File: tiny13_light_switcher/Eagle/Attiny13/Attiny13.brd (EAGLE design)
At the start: 80 x 85 mm, 39 parts, among them Q4 2N7000, Q5 2N7000, Q6 2N7000, U1 ATTiny13, U2 ATTiny85

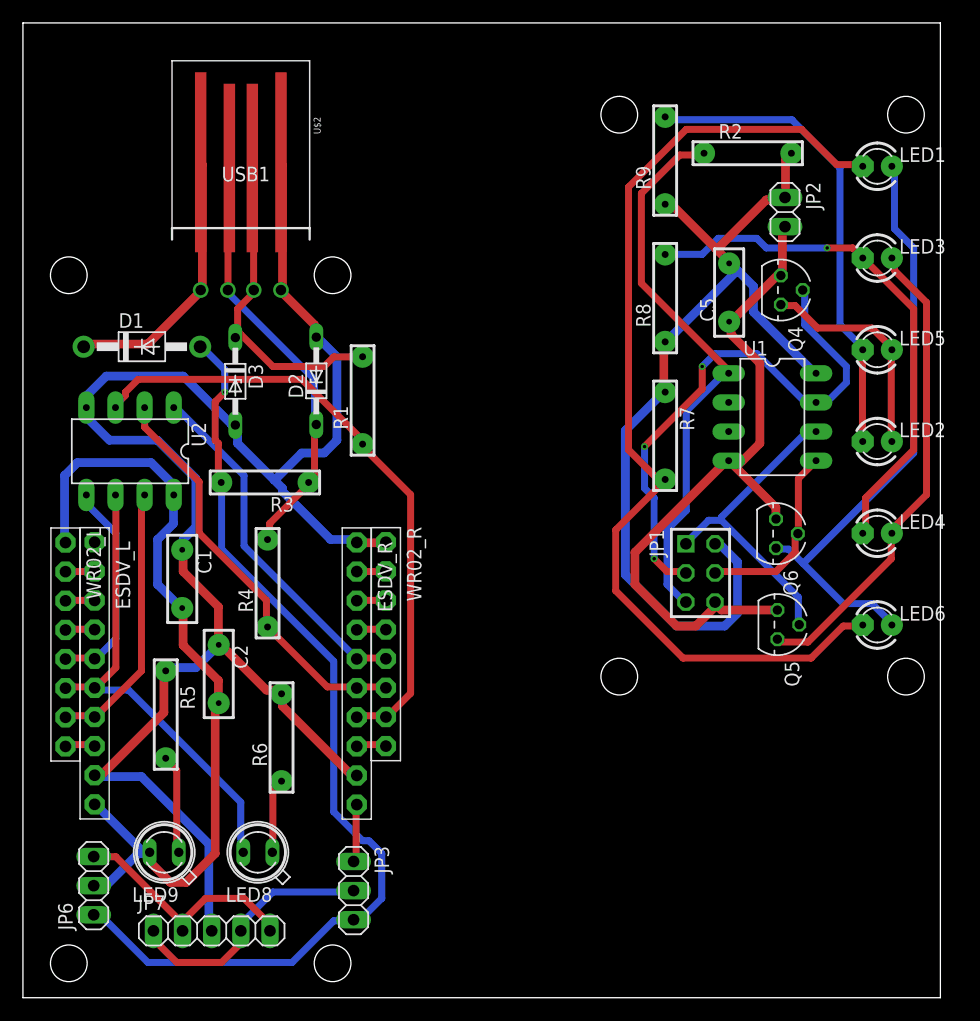
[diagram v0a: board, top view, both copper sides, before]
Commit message: Fix Wiring.
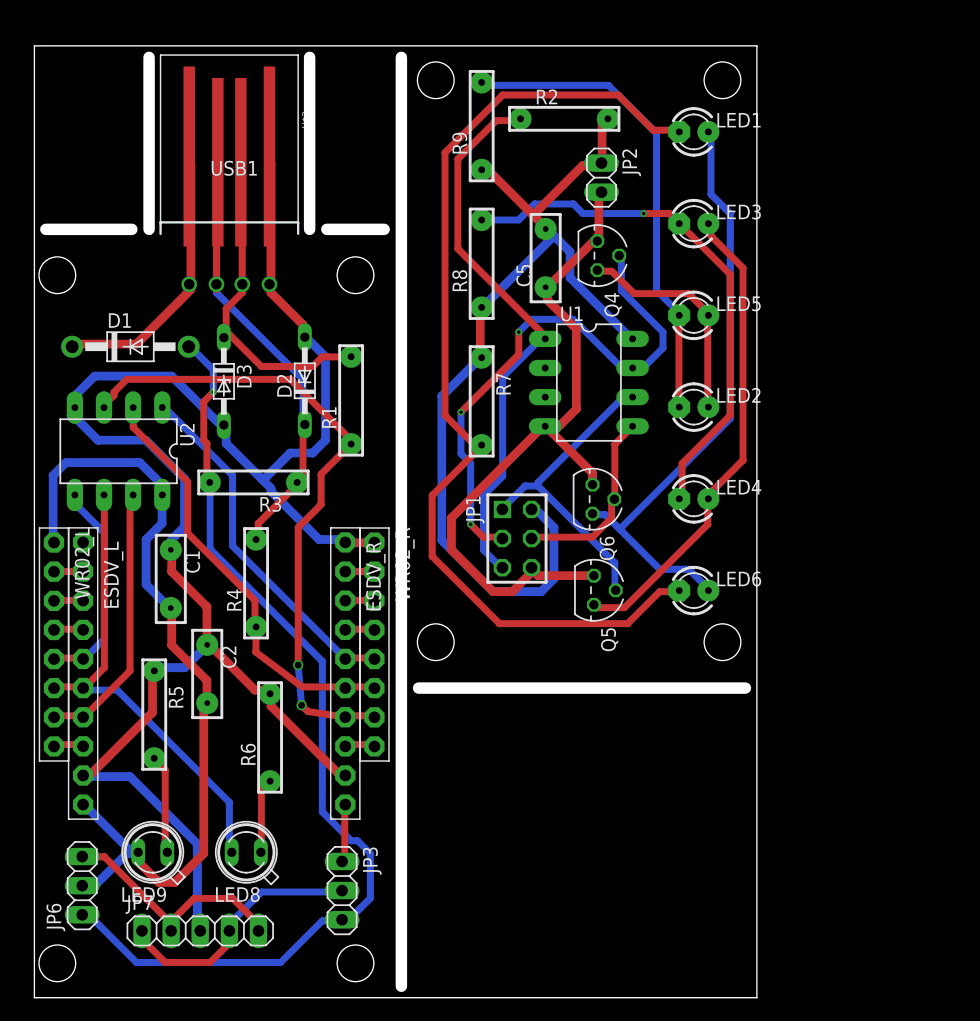
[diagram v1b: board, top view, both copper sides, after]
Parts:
- moved Q6 16.3 mm to (49.7, 43.5)
- moved C5 16.3 mm to (45.6, 64.5)
- moved JP1 16.3 mm to (43.1, 40.0)
- moved JP2 16.3 mm to (50.5, 71.5)
- moved LED1 16.3 mm to (58.5, 75.5)
- moved LED2 16.3 mm to (58.5, 51.5)
- moved LED3 16.3 mm to (58.5, 67.5)
- moved LED4 16.3 mm to (58.5, 43.5)
- moved LED5 16.3 mm to (58.5, 59.5)
- moved LED6 16.3 mm to (58.5, 35.5)
- moved Q4 16.3 mm to (50.1, 64.7)
- moved R2 16.3 mm to (47.2, 76.6)
- moved R7 16.3 mm to (40.0, 52.0)
- moved R8 16.3 mm to (40.0, 64.0)
- moved R9 16.3 mm to (40.0, 76.0)
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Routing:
- net N$11: track 54.6 -> 56.9 mm, vias 0 -> 2
- net N$19: track 28.1 -> 29.5 mm
- net N$4: track 37.6 -> 39.0 mm
- net N$1: track 23.7 -> 25.0 mm
- net N$3: track 36.2 -> 37.3 mm
- net AGND: track 152.4 -> 153.2 mm
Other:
- board size 80 x 85 mm -> 63 x 83 mm
